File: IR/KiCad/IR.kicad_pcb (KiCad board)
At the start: 2 copper layers, 26.9 x 15.2 mm, 5 parts, among them J1 Conn_01x06, M3 MountingHole_3.2mm_M3

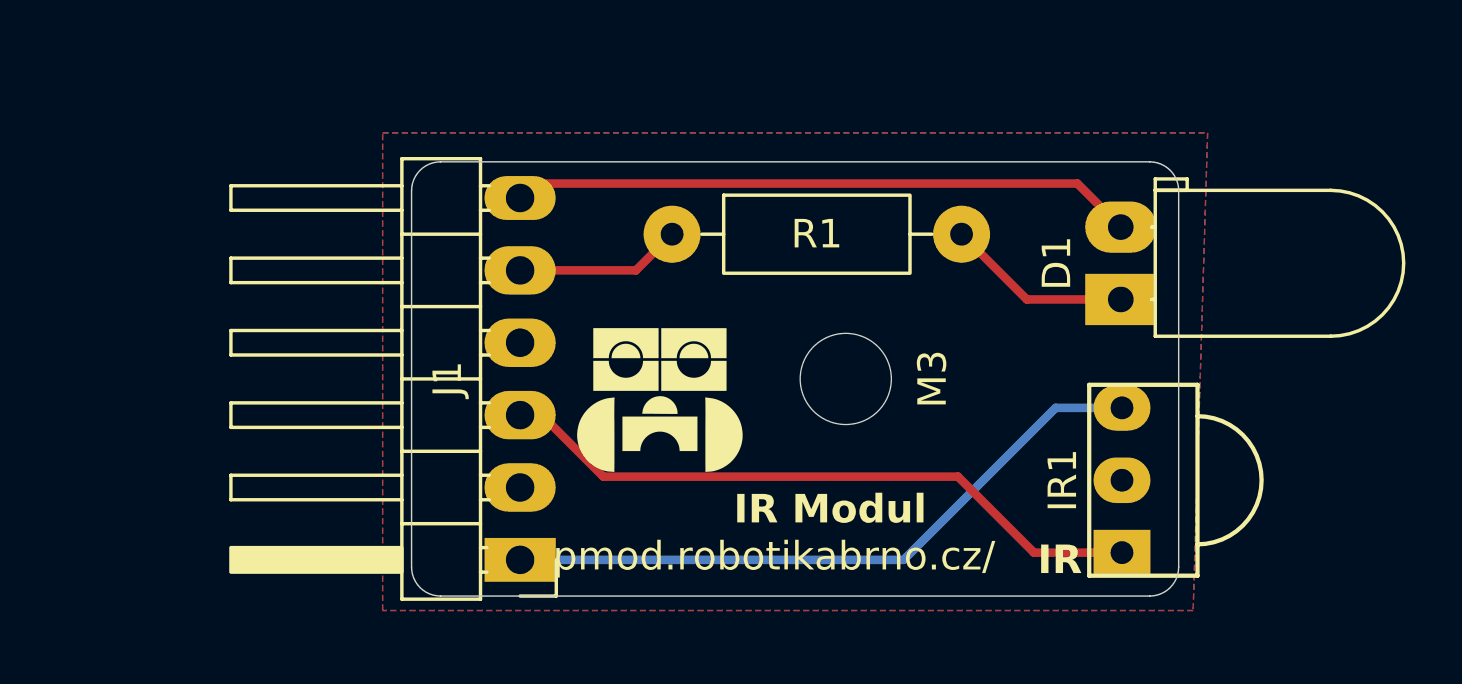
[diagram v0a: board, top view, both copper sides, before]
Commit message: Deployed de0c2bf with MkDocs version: 1.6.0
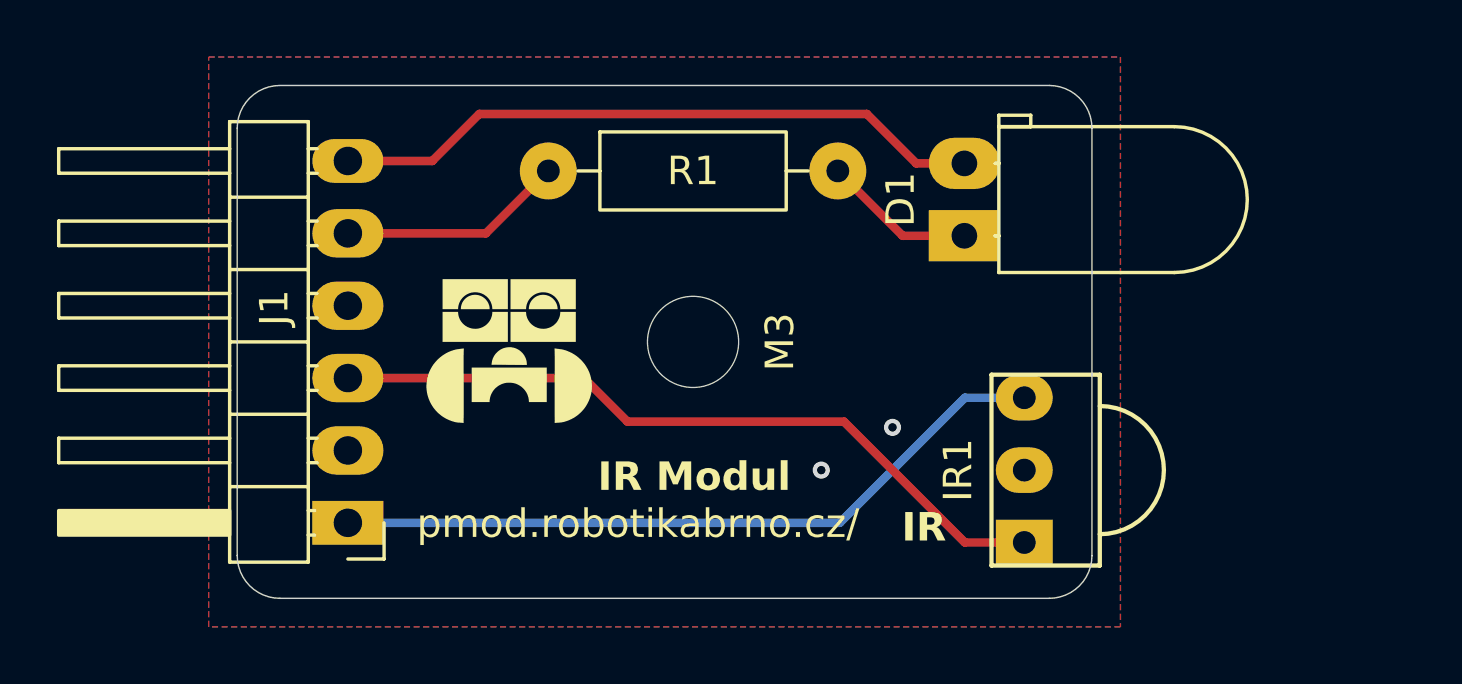
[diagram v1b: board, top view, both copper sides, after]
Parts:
- D1: value SFH4550 -> IR
- moved J1 6.18 mm to (68.9, 55.9)
- moved D1 5.93 mm to (90.5, 45.8)
- moved M3 5.52 mm to (81.0, 49.5)
- moved R1 4.88 mm to (75.9, 43.5)
- moved IR1 3.45 mm to (92.6, 54.0)
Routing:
- net RX: track 23.1 -> 26.1 mm
- net TX: track 5.86 -> 7.94 mm
- net +3.3V: track 23.8 -> 25.6 mm
- net GND: track 1.37 -> 0.00 mm, vias 0 -> 2
- net Net-(D1-K): track 6.54 -> 5.38 mm
- net CLK: track 21.9 -> 23.0 mm
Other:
- board size 26.9 x 15.2 mm -> 30 x 18 mm

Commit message: Deployed d972a79 with MkDocs version: 1.6.0
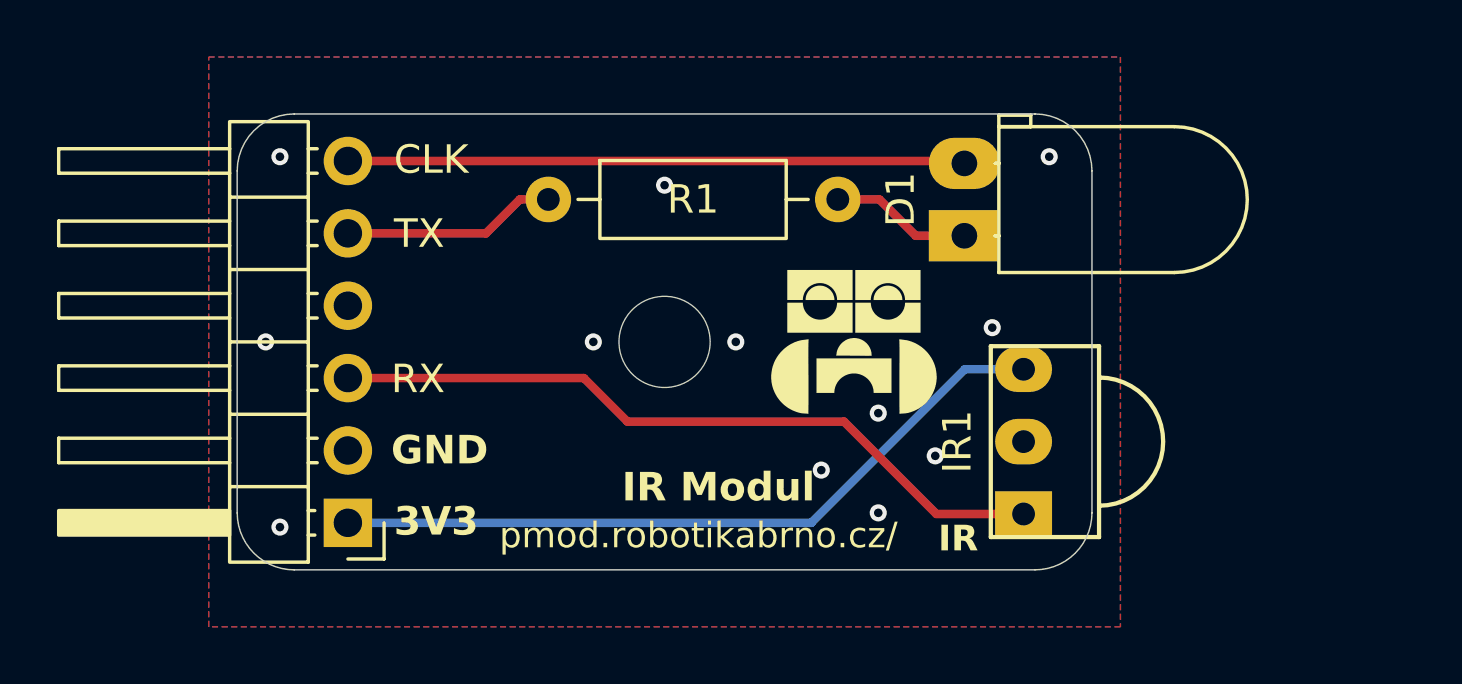
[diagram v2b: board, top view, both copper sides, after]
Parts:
- R1: value 180 -> 100
- moved IR1 1.00 mm to (92.6, 53.0)
- moved M3 1.00 mm to (80.0, 49.5)
- moved R1 1.00 mm to (75.9, 44.5)
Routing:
- net CLK: track 23.0 -> 21.7 mm
- net GND: vias 2 -> 12
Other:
- board size 30 x 18 mm -> 30 x 16 mm
- board text added: "16mm"
- board text added: "30mm"
- board text added: "3V3"
- board text added: "CLK"
- board text added: "GND"
- board text added: "RX"
- board text added: "TX"
